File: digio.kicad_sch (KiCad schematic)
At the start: 42 parts, among them J25 Conn_01x08, J26 Conn_01x08, J27 Conn_01x08, J28 Conn_01x08, J29 Conn_01x04, J30 Conn_01x04, U18 TCA9535PWR(UMW), U19 TCA9535PWR(UMW)

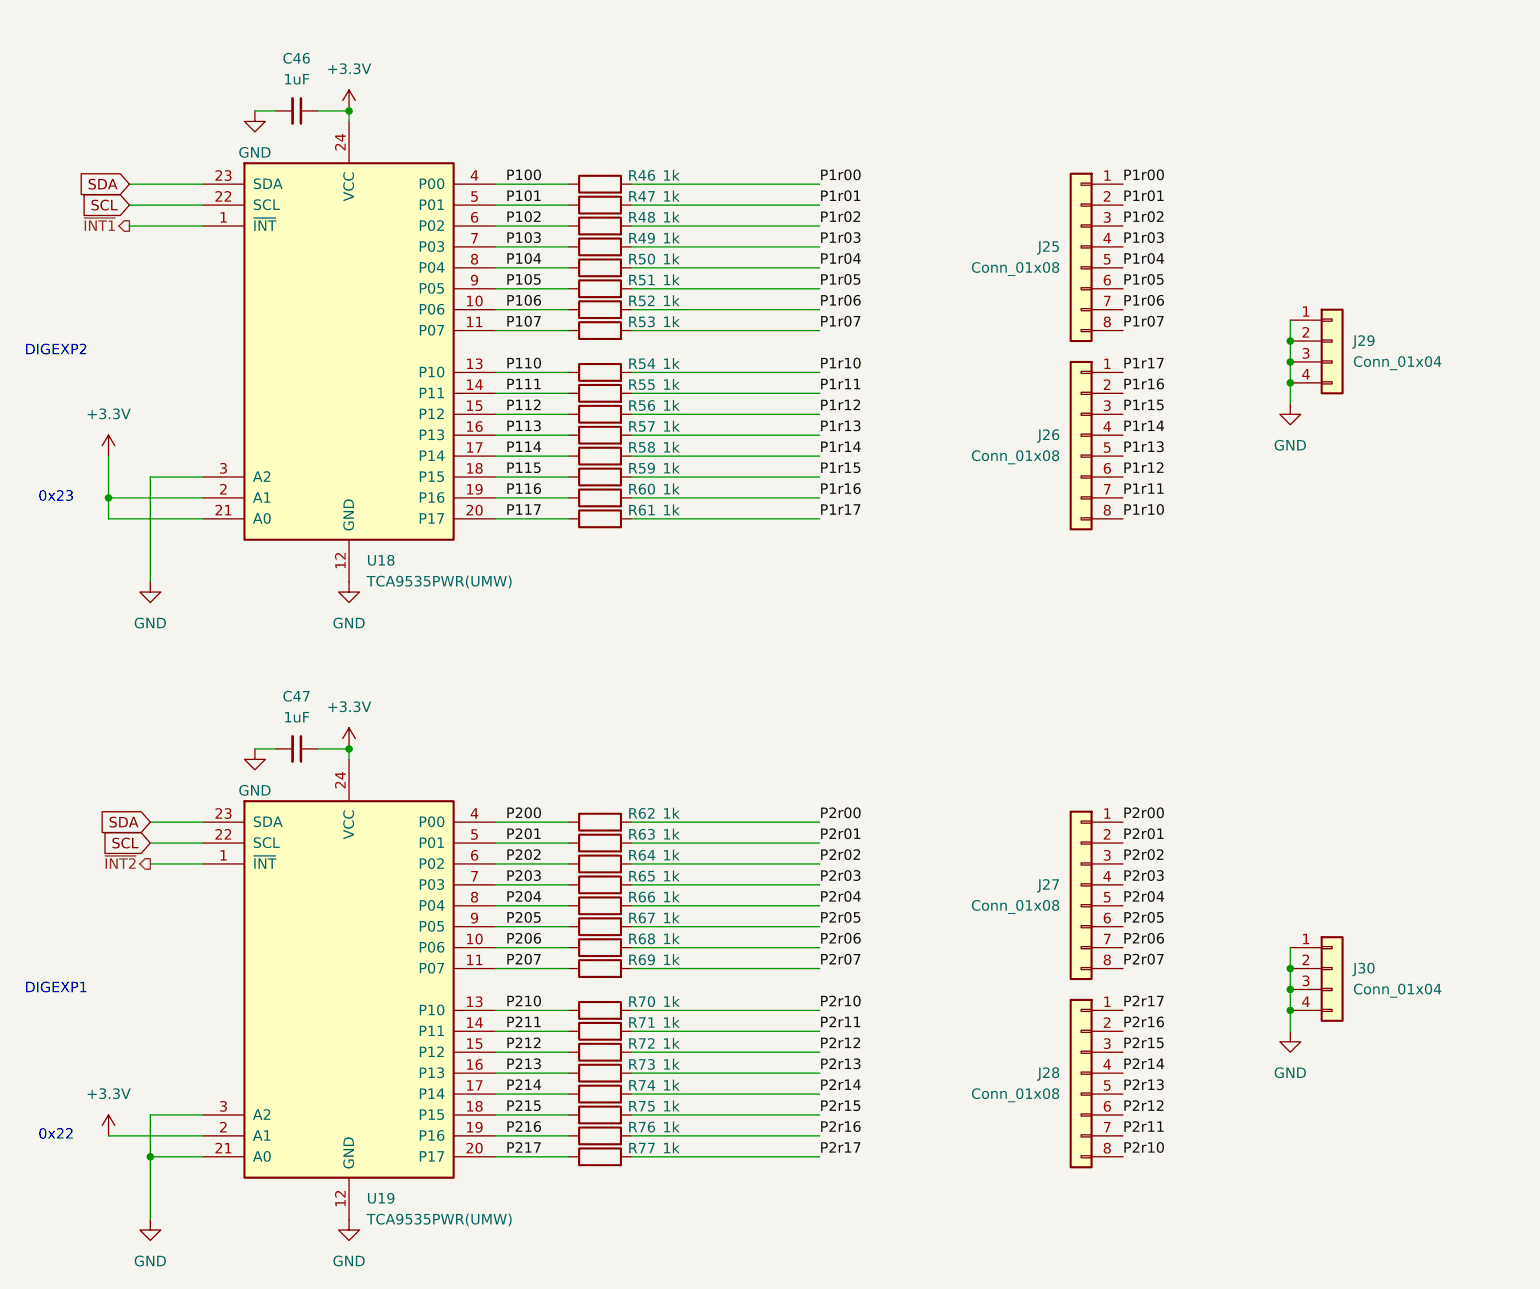
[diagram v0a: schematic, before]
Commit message: Assorted fixes
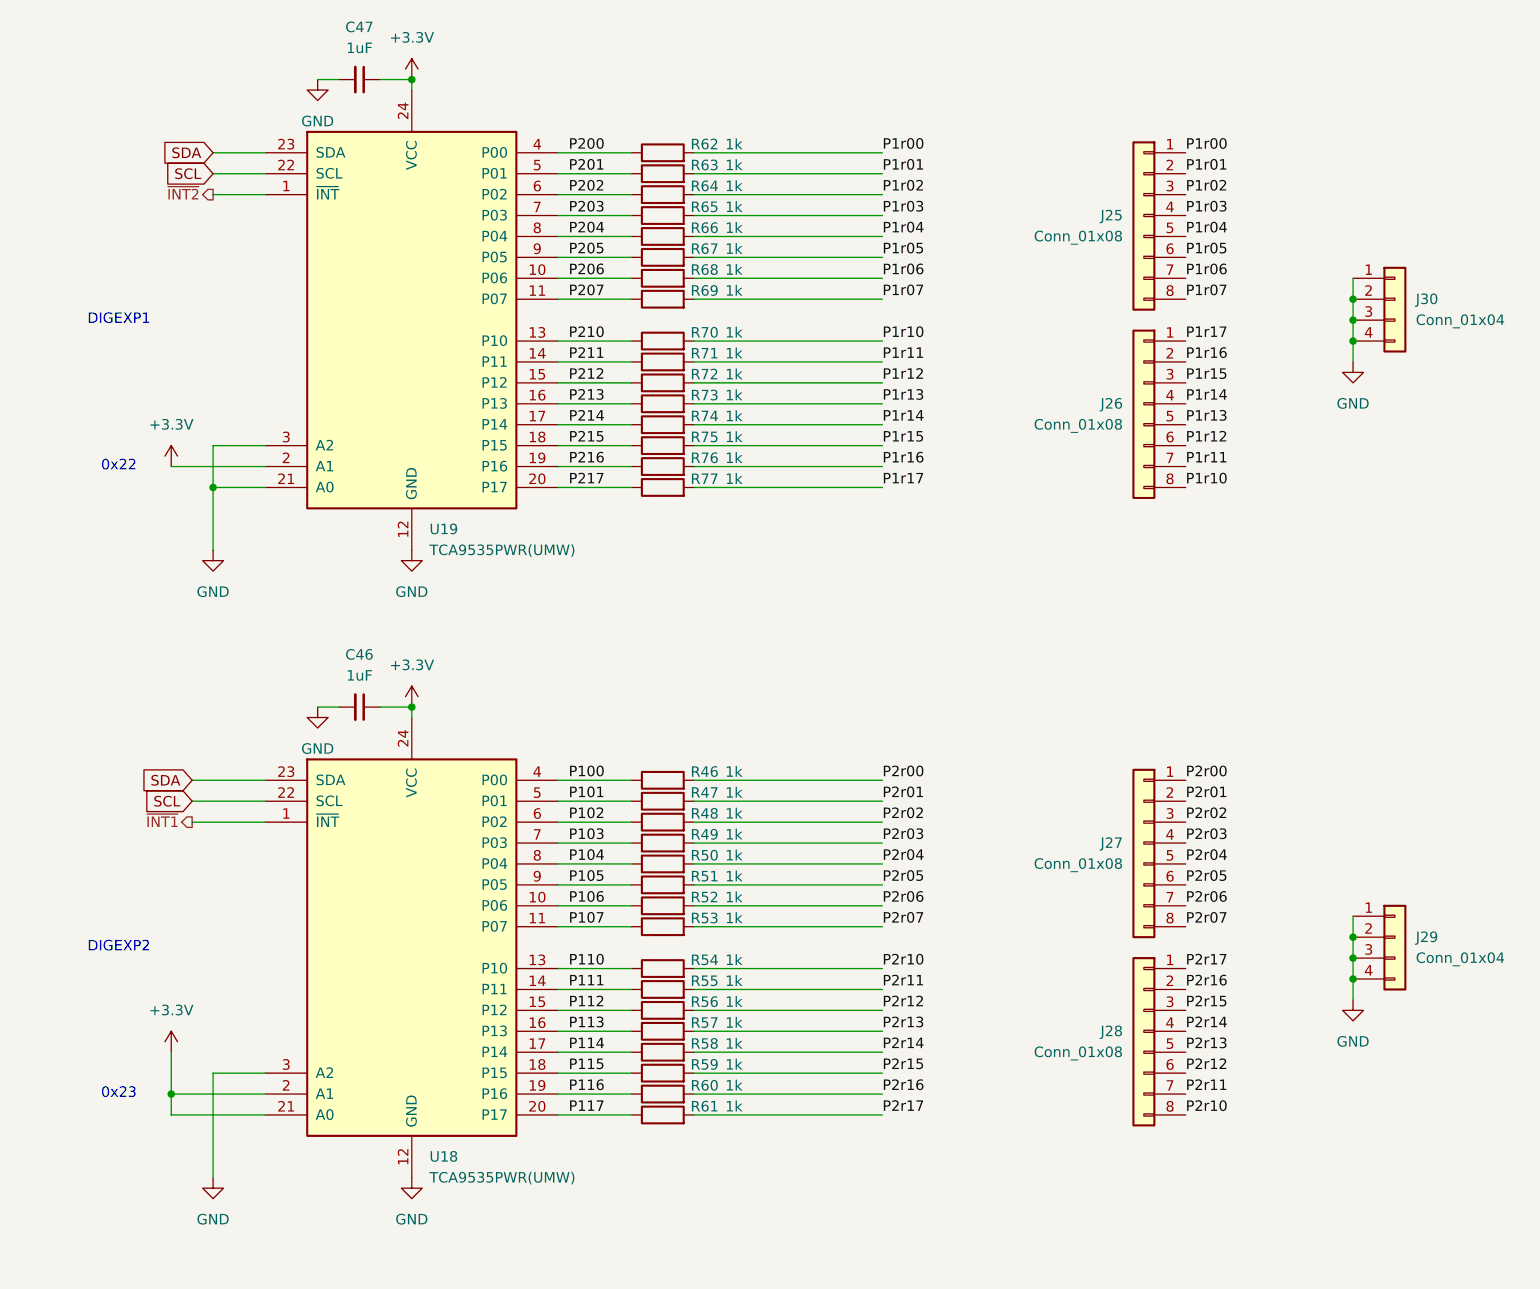
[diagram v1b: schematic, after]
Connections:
- net P1r00: now also R62.2; no longer R46.2
- net P1r01: now also R63.2; no longer R47.2
- net P1r02: now also R64.2; no longer R48.2
- net P1r03: now also R65.2; no longer R49.2
- net P1r04: now also R66.2; no longer R50.2
- net P1r05: now also R67.2; no longer R51.2
- net P1r06: now also R68.2; no longer R52.2
- net P1r07: now also R69.2; no longer R53.2
- net P1r10: now also R70.2; no longer R54.2
- net P1r11: now also R71.2; no longer R55.2
- net P1r12: now also R72.2; no longer R56.2
- net P1r13: now also R73.2; no longer R57.2
- net P1r14: now also R74.2; no longer R58.2
- net P1r15: now also R75.2; no longer R59.2
- net P1r16: now also R76.2; no longer R60.2
- net P1r17: now also R77.2; no longer R61.2
- net P2r00: now also R46.2; no longer R62.2
- net P2r01: now also R47.2; no longer R63.2
- net P2r02: now also R48.2; no longer R64.2
- net P2r03: now also R49.2; no longer R65.2
- net P2r04: now also R50.2; no longer R66.2
- net P2r05: now also R51.2; no longer R67.2
- net P2r06: now also R52.2; no longer R68.2
- net P2r07: now also R53.2; no longer R69.2
- net P2r10: now also R54.2; no longer R70.2
- net P2r11: now also R55.2; no longer R71.2
- net P2r12: now also R56.2; no longer R72.2
- net P2r13: now also R57.2; no longer R73.2
- net P2r14: now also R58.2; no longer R74.2
- net P2r15: now also R59.2; no longer R75.2
- net P2r16: now also R60.2; no longer R76.2
- net P2r17: now also R61.2; no longer R77.2
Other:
- moved on the sheet: C46, C47, J25, J26, J27, J28, J29, J30, R46, R47, R48, R49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
